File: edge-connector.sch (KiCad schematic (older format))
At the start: 3 parts, among them J5 SFF-TA-1002-4C+

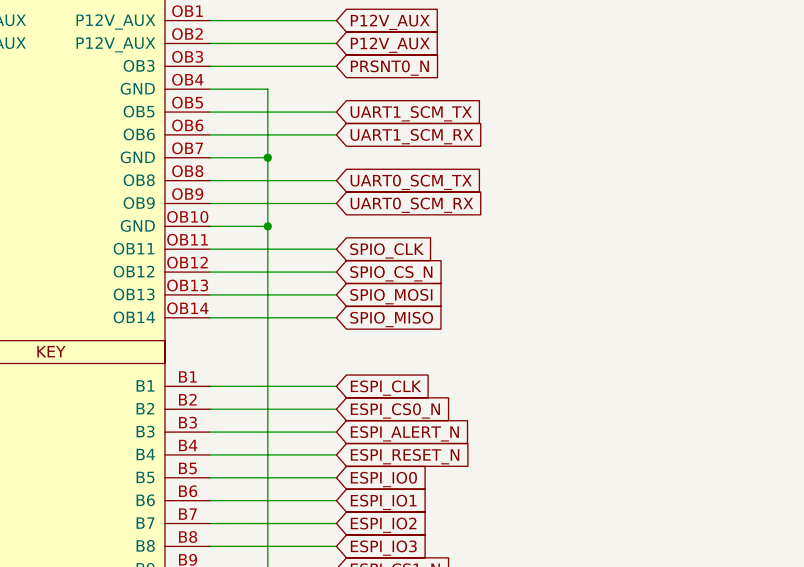
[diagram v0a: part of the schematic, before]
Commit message: Typo fix
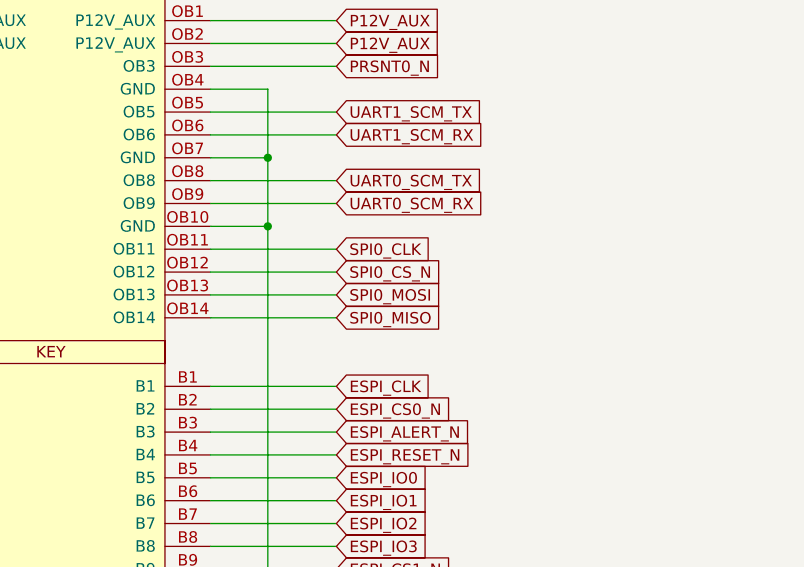
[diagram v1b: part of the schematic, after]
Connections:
- net SPIO_CLK renamed SPI0_CLK
- net SPIO_CS_N renamed SPI0_CS_N
- net SPIO_MISO renamed SPI0_MISO
- net SPIO_MOSI renamed SPI0_MOSI
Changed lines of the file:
@@
 UART0_SCM_RX
 Text GLabel 9125 2525 2    50   Input ~ 0
-SPIO_CLK
+SPI0_CLK
 Text GLabel 9125 2625 2    50   Input ~ 0
-SPIO_CS_N
+SPI0_CS_N
 Text GLabel 9125 2725 2    50   Input ~ 0
-SPIO_MOSI
+SPI0_MOSI
 Text GLabel 9125 2825 2    50   Input ~ 0
-SPIO_MISO
+SPI0_MISO
 Text GLabel 9125 3125 2    50   Input ~ 0
 ESPI_CLK
